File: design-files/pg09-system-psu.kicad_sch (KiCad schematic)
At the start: 3 parts, among them J1 ATX-24, J802 Power Switch

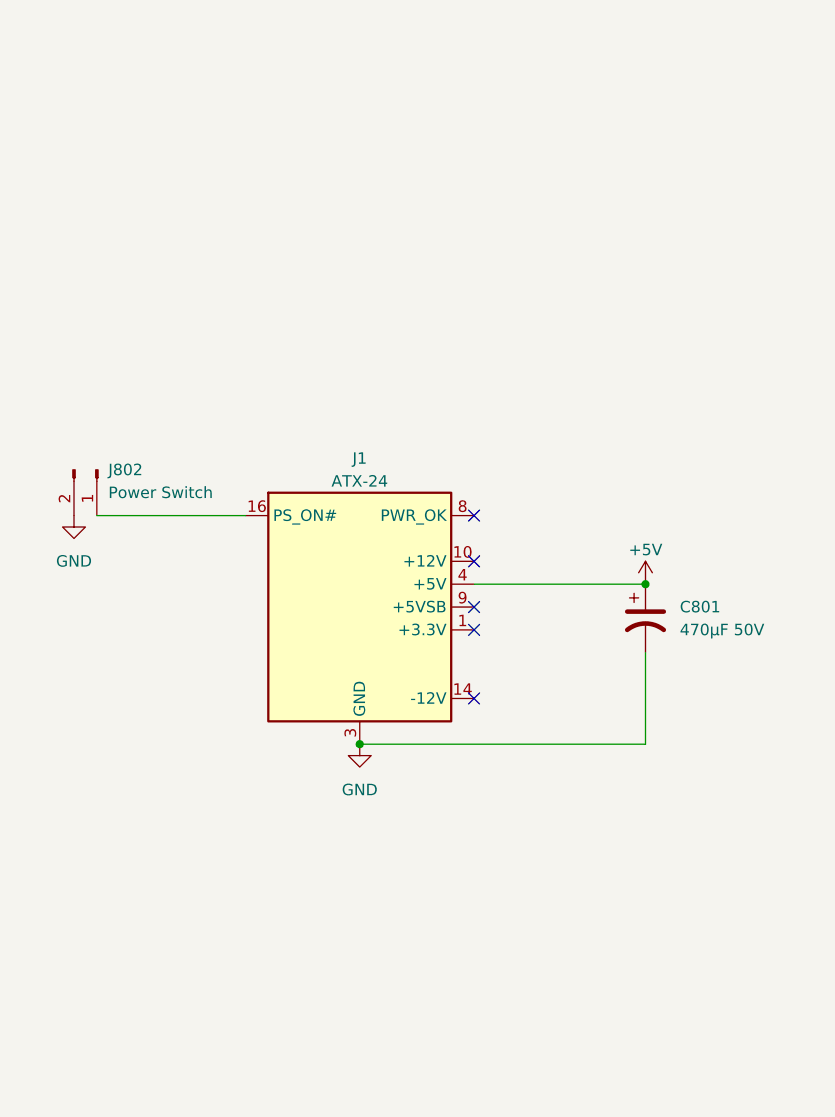
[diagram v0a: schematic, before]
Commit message: Add an Adafruit Metro Mini to act as a PSU controller.
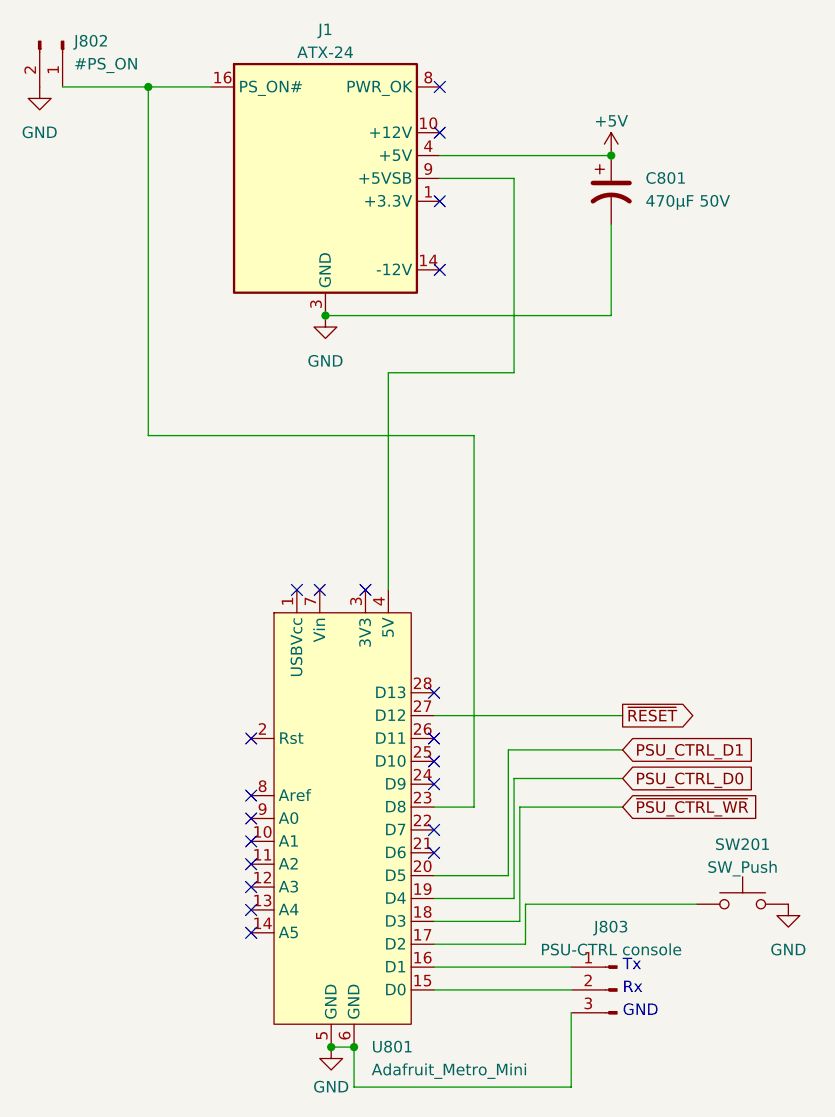
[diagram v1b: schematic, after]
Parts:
- added J803: PSU-CTRL console, Connector_PinHeader_2.54mm:PinHeader_1x03_P2.54mm_Vertical, symbol Connector:Conn_01x03_Pin
- added SW201: SW_Push, Button_Switch_THT:SW_PUSH_6mm, symbol Switch:SW_Push
- added U801: Adafruit_Metro_Mini, Package_DIP:DIP-28_W15.24mm_Socket, symbol jrt-Arduino:Adafruit_Metro_Mini
- J802: value Power Switch -> #PS_ON
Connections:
- net GND: now also J803.3 (Pin_3), SW201.2, U801.5 (GND), U801.6 (GND)
- net at J1.16 (PS_ON#), J802.1 (Pin_1): now also U801.23 (D8)
- net at J1.9 (+5VSB): now also U801.4 (5V)
- new net: J803.1 (Pin_1), U801.16 (D1)
- new net: J803.2 (Pin_2), U801.15 (D0)
- new net: SW201.1, U801.17 (D2)
- new net PSU_CTRL_D0: U801.19 (D4)
- new net PSU_CTRL_D1: U801.20 (D5)
- new net ~{PSU_CTRL_WR}: U801.18 (D3)
- new net ~{RESET}: U801.27 (D12)
- no-connect marks 5 -> 21
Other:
- note added: "GND"
- note added: "Rx"
- note added: "Tx"
- moved on the sheet: C801, J1, J802
